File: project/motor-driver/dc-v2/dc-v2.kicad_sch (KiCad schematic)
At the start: 6 parts, among them J1 Power, Q1 PMOS

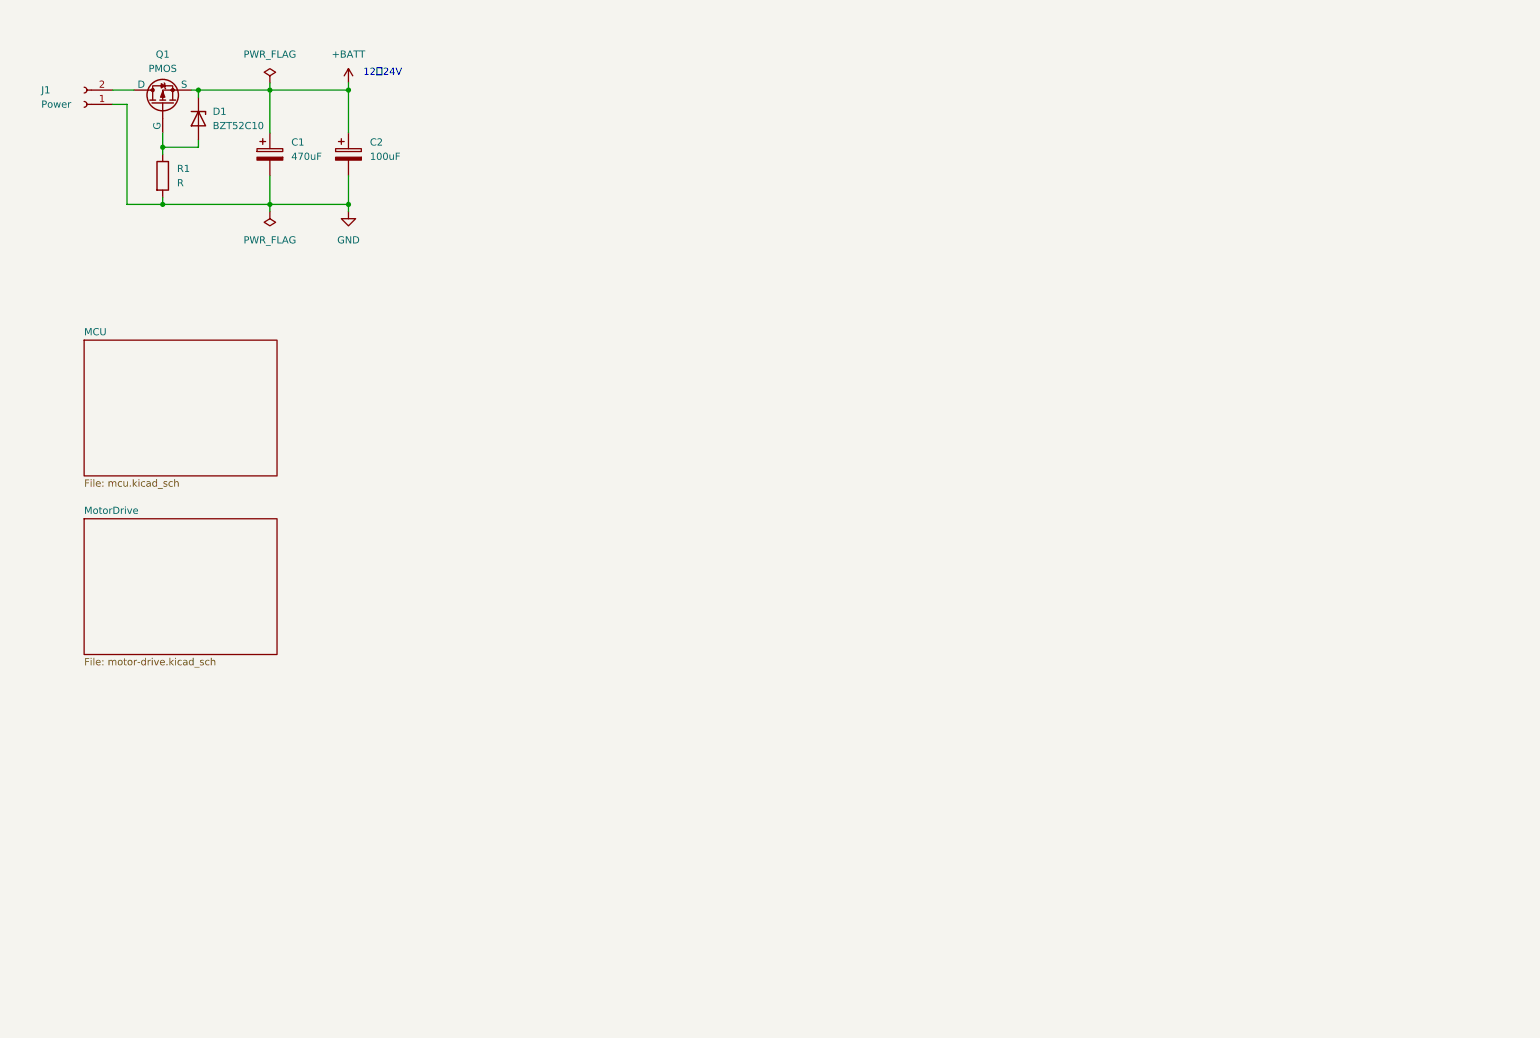
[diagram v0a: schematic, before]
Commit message: 2025/10/14/08:57
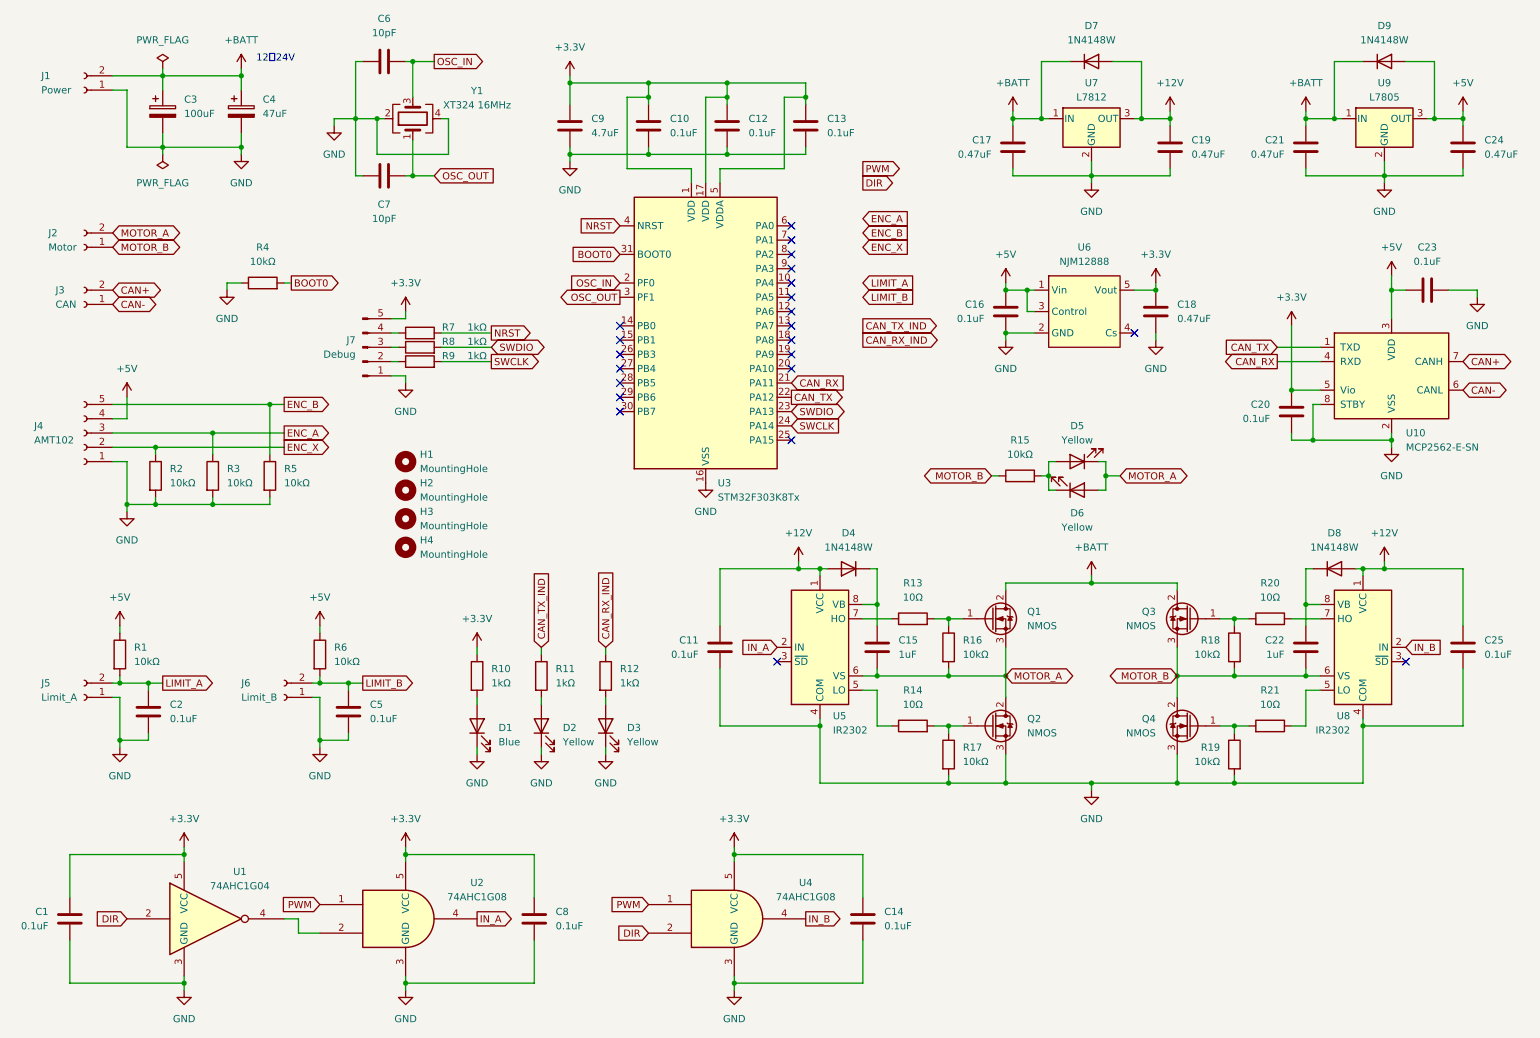
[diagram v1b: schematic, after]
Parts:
- removed D1: BZT52C10, symbol Device:D_Zener
- removed Q1: PMOS, Package_TO_SOT_SMD:TO-252-2, symbol Simulation_SPICE:PMOS
- added C1, C10, C11, C12, C13, C14, C16, C2, C20, C23, C25, C5, C8: 0.1uF, Capacitor_SMD:C_0603_1608Metric, symbol Device:C
- added C15, C22: 1uF, Capacitor_SMD:C_0805_2012Metric, symbol Device:C
- added C17, C18, C19, C21, C24: 0.47uF, Capacitor_SMD:C_0603_1608Metric, symbol Device:C
- added C6, C7: 10pF, Capacitor_SMD:C_0603_1608Metric, symbol Device:C
- added C9: 4.7uF, Capacitor_SMD:C_0603_1608Metric, symbol Device:C
- added D1: Blue, LED_SMD:LED_0603_1608Metric, symbol Device:LED
- added D2, D3, D5, D6: Yellow, LED_SMD:LED_0603_1608Metric, symbol Device:LED
- added D4, D7, D8, D9: 1N4148W, Diode_SMD:D_SOD-123, symbol Diode:1N4148W
- added H1, H2, H3, H4: MountingHole, MountingHole:MountingHole_3.2mm_M3, symbol Mechanical:MountingHole
- added J2: Motor, Connector_AMASS:AMASS_XT30PW-F_1x02_P2.50mm_Horizontal, symbol Connector:Conn_01x02_Socket
- added J3: CAN, Connector_JST:JST_XA_S02B-XASK-1N-BN_1x02_P2.50mm_Horizontal, symbol Connector:Conn_01x02_Socket
- added J4: AMT102, Connector_JST:JST_XH_S5B-XH-A_1x05_P2.50mm_Horizontal, symbol Connector:Conn_01x05_Socket
- added J5: Limit_A, Connector_JST:JST_XH_S2B-XH-A_1x02_P2.50mm_Horizontal, symbol Connector:Conn_01x02_Socket
- added J6: Limit_B, Connector_JST:JST_XH_S2B-XH-A_1x02_P2.50mm_Horizontal, symbol Connector:Conn_01x02_Socket
- added J7: Debug, Connector_PinSocket_2.54mm:PinSocket_1x05_P2.54mm_Horizontal, symbol Connector:Conn_01x05_Pin
- added Q1, Q2, Q3, Q4: NMOS, Package_TO_SOT_SMD:TO-252-2, symbol Transistor_FET_Other:Q_NMOS_Depletion_GDS
- added R10, R11, R12, R7, R8, R9: 1kΩ, Resistor_SMD:R_0603_1608Metric, symbol Device:R
- added R13, R14, R20, R21: 10Ω, Resistor_SMD:R_0603_1608Metric, symbol Device:R
- added R15, R16, R17, R18, R19, R2, R3, R4, R5, R6: 10kΩ, Resistor_SMD:R_0603_1608Metric, symbol Device:R
- added U1: 74AHC1G04, Package_TO_SOT_SMD:SOT-23-5, symbol 74xGxx:74AHC1G04
- added U10: MCP2562-E-SN, Package_SO:SOIC-8_3.9x4.9mm_P1.27mm, symbol Interface_CAN_LIN:MCP2562-E-SN
- added U2, U4: 74AHC1G08, Package_TO_SOT_SMD:SOT-23-5, symbol 74xGxx:74AHC1G08
- added U3: STM32F303K8Tx, Package_QFP:LQFP-32_7x7mm_P0.8mm, symbol MCU_ST_STM32F3:STM32F303K8Tx
- added U5, U8: IR2302, Package_SO:SOIC-8_3.9x4.9mm_P1.27mm, symbol Driver_FET:IR2302
- added U6: NJM12888, Package_TO_SOT_SMD:SOT-23-5, symbol JRC_Regulator_Linear:NJM12888F33
- added U7: L7812, Package_TO_SOT_SMD:TO-252-2, symbol Regulator_Linear:L7812
- added U9: L7805, Package_TO_SOT_SMD:TO-252-2, symbol Regulator_Linear:L7805
- added Y1: XT324 16MHz, Crystal:Crystal_SMD_3225-4Pin_3.2x2.5mm, symbol Device:Crystal_GND24
- C3: renamed from C1; value 470uF -> 100uF; footprint (none) -> Capacitor_THT:CP_Radial_D8.0mm_P3.50mm
- C4: renamed from C2; value 100uF -> 47uF; footprint (none) -> Capacitor_THT:CP_Radial_D6.3mm_P2.50mm
- R1: value R -> 10kΩ; footprint (none) -> Resistor_SMD:R_0603_1608Metric
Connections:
- net +BATT: now also J1.2 (Pin_2), C17.1, C21.1, D7.1 (K), D9.1 (K), Q1.2 (D), Q3.2 (D), U7.1 (IN), U9.1 (IN)
- net GND: now also C1.2, C10.2, C11.2, C12.2, C13.2, C14.2, C16.2, C17.2, C18.2, C19.2, C2.2, C20.1, C21.2, C23.1, C24.2, C25.2, C5.2, C6.1, C7.1, C8.2, C9.2, D1.1 (K), D2.1 (K), D3.1 (K), J4.1 (Pin_1), J5.1 (Pin_1), J6.1 (Pin_1), J7.1 (Pin_1), Q2.3 (S), Q4.3 (S), R17.2, R19.2, R2.2, R3.2, R4.1, R5.2, U1.3 (GND), U10.2 (VSS), U10.8 (STBY), U2.3 (GND), U3.16 (VSS), U3.32 (VSS), U4.3 (GND), U5.4 (COM), U6.2 (GND), U7.2 (GND), U8.4 (COM), U9.2 (GND), Y1.2, Y1.4; no longer R1.2
- net +5V: now reaches R1.1
- net +5V: now also C16.1, C23.2, C24.1, D9.2 (A), J4.4 (Pin_4), R6.1, U10.3 (VDD), U6.1 (Vin), U6.3 (Control), U9.3 (OUT)
- new net: R20.1, U8.7 (HO)
- new net: Q3.1 (G), R18.1, R20.2
- new net: Q1.1 (G), R13.2, R16.1
- new net: J7.4 (Pin_4), R7.1
- new net: C15.1, D4.1 (K), U5.8 (VB)
- new net: J7.2 (Pin_2), R9.1
- new net: J7.3 (Pin_3), R8.1
- new net: Q4.1 (G), R19.1, R21.2
- new net: R21.1, U8.5 (LO)
- new net: R13.1, U5.7 (HO)
- new net: Q2.1 (G), R14.2, R17.1
- new net: C22.1, D8.1 (K), U8.8 (VB)
- new net: D5.2 (A), D6.1 (K), R15.2
- new net: D2.2 (A), R11.2
- new net: U1.4, U2.2
- new net: D3.2 (A), R12.2
- new net: R14.1, U5.5 (LO)
- new net: D1.2 (A), R10.2
- new net +12V: C11.1, C19.1, C25.1, D4.2 (A), D7.2 (A), D8.2 (A), U5.1 (VCC), U7.3 (OUT), U8.1 (VCC)
- new net +3.3V: C1.1, C10.1, C12.1, C13.1, C14.1, C18.1, C20.2, C8.1, C9.1, J7.5 (Pin_5), R10.1, U1.5 (VCC), U10.5 (Vio), U2.5 (VCC), U3.1 (VDD), U3.17 (VDD), U3.5 (VDDA), U4.5 (VCC), U6.5 (Vout)
- new net BOOT0: R4.2, U3.31 (BOOT0)
- new net CAN+: J3.2 (Pin_2), U10.7 (CANH)
- new net CAN-: J3.1 (Pin_1), U10.6 (CANL)
- new net CAN_RX: U10.4 (RXD), U3.21 (PA11)
- new net CAN_RX_IND: R12.1
- new net CAN_TX: U10.1 (TXD), U3.22 (PA12)
- new net CAN_TX_IND: R11.1
- new net DIR: U1.2, U4.2
- new net ENC_A: J4.3 (Pin_3), R3.1
- new net ENC_B: J4.5 (Pin_5), R5.1
- new net ENC_X: J4.2 (Pin_2), R2.1
- new net IN_A: U2.4, U5.2 (IN)
- new net IN_B: U4.4, U8.2 (IN)
- new net LIMIT_A: C2.1, J5.2 (Pin_2), R1.2
- new net LIMIT_B: C5.1, J6.2 (Pin_2), R6.2
- new net MOTOR_A: C15.2, D5.1 (K), D6.2 (A), J2.2 (Pin_2), Q1.3 (S), Q2.2 (D), R16.2, U5.6 (VS)
- new net MOTOR_B: C22.2, J2.1 (Pin_1), Q3.3 (S), Q4.2 (D), R15.1, R18.2, U8.6 (VS)
- new net NRST: R7.2, U3.4 (NRST)
- new net OSC_IN: C6.2, U3.2 (PF0), Y1.3
- new net OSC_OUT: C7.2, U3.3 (PF1), Y1.1
- new net PWM: U2.1, U4.1
- new net SWCLK: R9.2, U3.24 (PA14)
- new net SWDIO: R8.2, U3.23 (PA13)
- no-connect marks 0 -> 22
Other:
- removed sheet MCU
- removed sheet MotorDrive
- moved on the sheet: C3, C4, J1
